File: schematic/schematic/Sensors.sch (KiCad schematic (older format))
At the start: 18 parts, among them J11 Conn_01x07, J12 Conn_01x07, J13 Conn_01x04, J14 Conn_01x04, U10 MPU-9250, U11 MPU-9250, U9 INA219AIDCNR

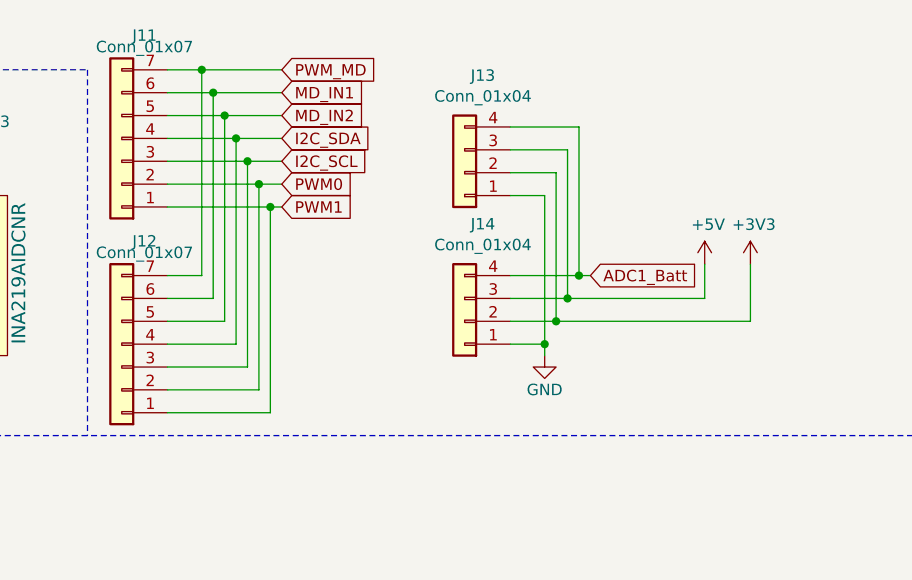
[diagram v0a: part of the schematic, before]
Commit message: 地獄の配線
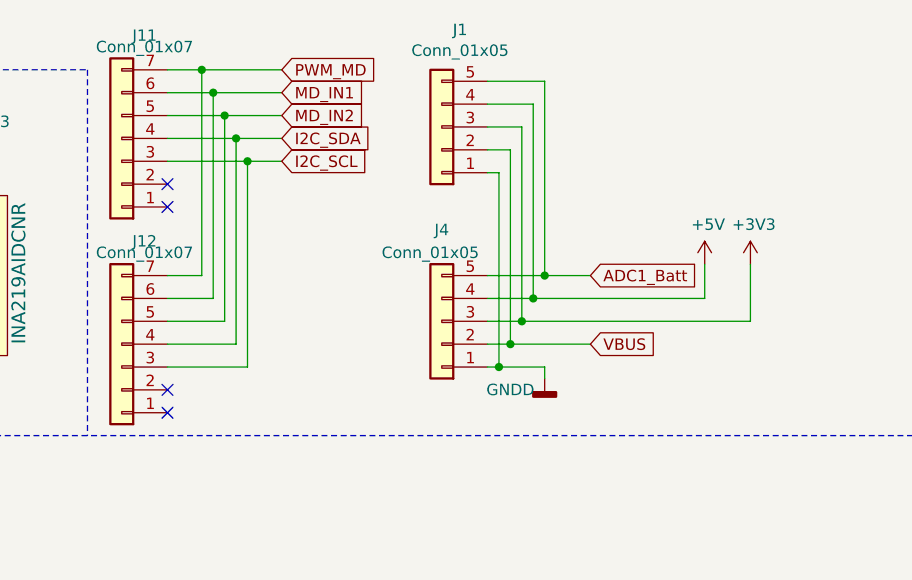
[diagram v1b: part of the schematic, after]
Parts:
- removed J13, J14: Conn_01x04, Connector_PinSocket_2.54mm:PinSocket_1x04_P2.54mm_Vertical, symbol Connector_Generic:Conn_01x04
- added J1, J4: Conn_01x05, Connector_PinHeader_1.00mm:PinHeader_2x03_P1.00mm_Vertical_SMD, symbol Connector_Generic:Conn_01x05
- J11, J12: footprint Connector_PinSocket_2.54mm:PinSocket_1x07_P2.54mm_Vertical -> Connector_PinHeader_1.00mm:PinHeader_2x04_P1.00mm_Vertical_SMD
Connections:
- net +3V3: now also J1.3 (Pin_3), J4.3 (Pin_3)
- net +5V: now also J1.4 (Pin_4), J4.4 (Pin_4)
- net ADC1_Batt: now also J1.5 (Pin_5), J4.5 (Pin_5)
- net GNDD: now also J1.1 (Pin_1), J4.1 (Pin_1)
- net PWM0: no longer names the net of J11.2 (Pin_2)
- net PWM0: no longer J12.2 (Pin_2)
- net PWM1: no longer names the net of J11.1 (Pin_1)
- net PWM1: no longer J12.1 (Pin_1)
- new net VBUS: J1.2 (Pin_2), J4.2 (Pin_2)
- no-connect marks 10 -> 14
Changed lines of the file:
@@
 Text GLabel 3500 1100 2    50   Input ~ 0
 I2C_SCL
-$Comp
-L power:GND #PWR?
-U 1 1 5EC61195
-P 4650 1950
-AR Path="/5EC61195" Ref="#PWR?"  Part="1"
-AR Path="/5E247314/5EC61195" Ref="#PWR075"  Part="1"
-F 0 "#PWR075" H 4650 1700 50  0001 C CNN
-F 1 "GND" H 4650 1800 50  0000 C CNN
-F 2 "" H 4650 1950 50  0001 C CNN
-F 3 "" H 4650 1950 50  0001 C CNN
-	1    4650 1950
-	1    0    0    -1
-$EndComp
 Text GLabel 4850 1600 2    50   Input ~ 0
 ADC1_Batt
 Wire Wire Line
-	4650 1950 4650 1900
-$Comp
-L Connector_Generic:Conn_01x04 J14
-U 1 1 5ECB2FF3
-P 4300 1800
-F 0 "J14" H 4220 1375 50  0000 C CNN
-F 1 "Conn_01x04" H 4220 1466 50  0000 C CNN
-F 2 "Connector_PinSocket_2.54mm:PinSocket_1x04_P2.54mm_Vertical" H 4300 1800 50  0001 C CNN
-F 3 "~" H 4300 1800 50  0001 C CNN
-	1    4300 1800
-	-1   0    0    1
-$EndComp
-$Comp
-L Connector_Generic:Conn_01x04 J13
-U 1 1 5ECB3055
-P 4300 1150
-F 0 "J13" H 4220 725 50  0000 C CNN
-F 1 "Conn_01x04" H 4220 816 50  0000 C CNN
-F 2 "Connector_PinSocket_2.54mm:PinSocket_1x04_P2.54mm_Vertical" H 4300 1150 50  0001 C CNN
-F 3 "~" H 4300 1150 50  0001 C CNN
-	1    4300 1150
-	-1   0    0    1
-$EndComp
-Wire Wire Line
-	4500 1900 4650 1900
+	4650 2050 4650 2000
 $Comp
 L power:+3V3 #PWR077
@@
 	5350 1550 5350 1700
 Wire Wire Line
-	4650 1900 4650 1250
-Wire Wire Line
-	4650 1250 4500 1250
-Connection ~ 4650 1900
-Wire Wire Line
-	4500 1700 4750 1700
-Wire Wire Line
-	4500 1800 4700 1800
-Wire Wire Line
-	4500 1150 4700 1150
-Wire Wire Line
-	4700 1150 4700 1800
-Connection ~ 4700 1800
-Wire Wire Line
-	4500 1050 4750 1050
-Wire Wire Line
-	4750 1050 4750 1700
-Connection ~ 4750 1700
-Wire Wire Line
 	5550 1550 5550 1800
-Wire Wire Line
-	4750 1700 5350 1700
-Wire Wire Line
-	4700 1800 5550 1800
-Wire Wire Line
-	4500 950  4800 950
-Wire Wire Line
-	4800 950  4800 1600
-Wire Wire Line
-	4800 1600 4500 1600
-Wire Wire Line
-	4850 1600 4800 1600
-Connection ~ 4800 1600
-Text GLabel 3500 1200 2    50   Input ~ 0
-PWM0
-Text GLabel 3500 1300 2    50   Input ~ 0
-PWM1
 $Comp
 L Connector_Generic:Conn_01x07 J11
@@
 F 0 "J11" H 2700 550 50  0000 C CNN
 F 1 "Conn_01x07" H 2700 600 50  0000 C CNN
-F 2 "Connector_PinSocket_2.54mm:PinSocket_1x07_P2.54mm_Vertical" H 2800 1000 50  0001 C CNN
+F 2 "Connector_PinHeader_1.00mm:PinHeader_2x04_P1.00mm_Vertical_SMD" H 2800 1000 50  0001 C CNN
 F 3 "~" H 2800 1000 50  0001 C CNN
 	1    2800 1000
@@
 F 0 "J12" H 2700 1450 50  0000 C CNN
 F 1 "Conn_01x07" H 2700 1500 50  0000 C CNN
-F 2 "Connector_PinSocket_2.54mm:PinSocket_1x07_P2.54mm_Vertical" H 2800 1900 50  0001 C CNN
+F 2 "Connector_PinHeader_1.00mm:PinHeader_2x04_P1.00mm_Vertical_SMD" H 2800 1900 50  0001 C CNN
 F 3 "~" H 2800 1900 50  0001 C CNN
 	1    2800 1900
@@
 	3000 1100 3350 1100
 Wire Wire Line
-	3000 1200 3400 1200
-Wire Wire Line
 	3000 1600 3150 1600
 Wire Wire Line
@@
 Connection ~ 3350 1100
 Wire Wire Line
-	3400 1200 3400 2100
-Wire Wire Line
-	3400 2100 3000 2100
-Connection ~ 3400 1200
-Wire Wire Line
-	3000 1300 3450 1300
-Wire Wire Line
-	3400 1200 3500 1200
-Wire Wire Line
 	3350 1100 3500 1100
 Wire Wire Line
@@
 Wire Wire Line
 	3150 700  3500 700
-Wire Wire Line
-	3450 1300 3450 2200
-Wire Wire Line
-	3450 2200 3000 2200
-Connection ~ 3450 1300
-Wire Wire Line
-	3450 1300 3500 1300
 $Comp
 L Device:R_Small R29
@@
 	1    0    0    -1
 $EndComp
+$Comp
+L Connector_Generic:Conn_01x05 J4
+U 1 1 5EF1C02F
+P 4200 1800
+F 0 "J4" H 4200 1400 50  0000 C CNN
+F 1 "Conn_01x05" H 4250 1500 50  0000 C CNN
+F 2 "Connector_PinHeader_1.00mm:PinHeader_2x03_P1.00mm_Vertical_SMD" H 4200 1800 50  0001 C CNN
+F 3 "~" H 4200 1800 50  0001 C CNN
+	1    4200 1800
+	-1   0    0    1
+$EndComp
+Wire Wire Line
+	4400 1600 4650 1600
+Wire Wire Line
+	4400 1700 4600 1700
+Wire Wire Line
+	4400 1800 4550 1800
+Wire Wire Line
+	4400 1900 4500 1900
+Wire Wire Line
+	4400 2000 4450 2000
+$Comp
+L Connector_Generic:Conn_01x05 J1
+U 1 1 5EF40D9B
+P 4200 950
+F 0 "J1" H 4120 525 50  0000 C CNN
+F 1 "Conn_01x05" H 4120 616 50  0000 C CNN
+F 2 "Connector_PinHeader_1.00mm:PinHeader_2x03_P1.00mm_Vertical_SMD" H 4200 950 50  0001 C CNN
+F 3 "~" H 4200 950 50  0001 C CNN
+	1    4200 950
+	-1   0    0    1
+$EndComp
+Wire Wire Line
+	4400 1150 4450 1150
+Wire Wire Line
+	4450 1150 4450 2000
+Connection ~ 4450 2000
+Wire Wire Line
+	4450 2000 4650 2000
+Wire Wire Line
+	4500 1900 4500 1050
+Wire Wire Line
+	4500 1050 4400 1050
+Connection ~ 4500 1900
+Wire Wire Line
+	4500 1900 4850 1900
+Wire Wire Line
+	4400 950  4550 950
+Wire Wire Line
+	4550 950  4550 1800
+Connection ~ 4550 1800
+Wire Wire Line
+	4550 1800 5550 1800
+Wire Wire Line
+	4600 1700 4600 850
+Wire Wire Line
+	4600 850  4400 850
+Connection ~ 4600 1700
+Wire Wire Line
+	4600 1700 5350 1700
+Wire Wire Line
+	4400 750  4650 750
+Wire Wire Line
+	4650 750  4650 1600
+Connection ~ 4650 1600
+Wire Wire Line
+	4650 1600 4850 1600
+Text GLabel 4850 1900 2    50   Input ~ 0
+VBUS
+$Comp
+L power:GNDD #PWR?
+U 1 1 5EF5FD4C
+P 4650 2050
+AR Path="/5EF5FD4C" Ref="#PWR?"  Part="1"
+AR Path="/5E247314/5EF5FD4C" Ref="#PWR0101"  Part="1"
+F 0 "#PWR0101" H 4650 1800 50  0001 C CNN
+F 1 "GNDD" H 4500 2000 50  0000 C CNN
+F 2 "" H 4650 2050 50  0001 C CNN
+F 3 "" H 4650 2050 50  0001 C CNN
+	1    4650 2050
+	1    0    0    -1
+$EndComp
+NoConn ~ 3000 2100
+NoConn ~ 3000 2200
+NoConn ~ 3000 1300
+NoConn ~ 3000 1200
 Wire Bus Line
 	1550 5550 1550 5950

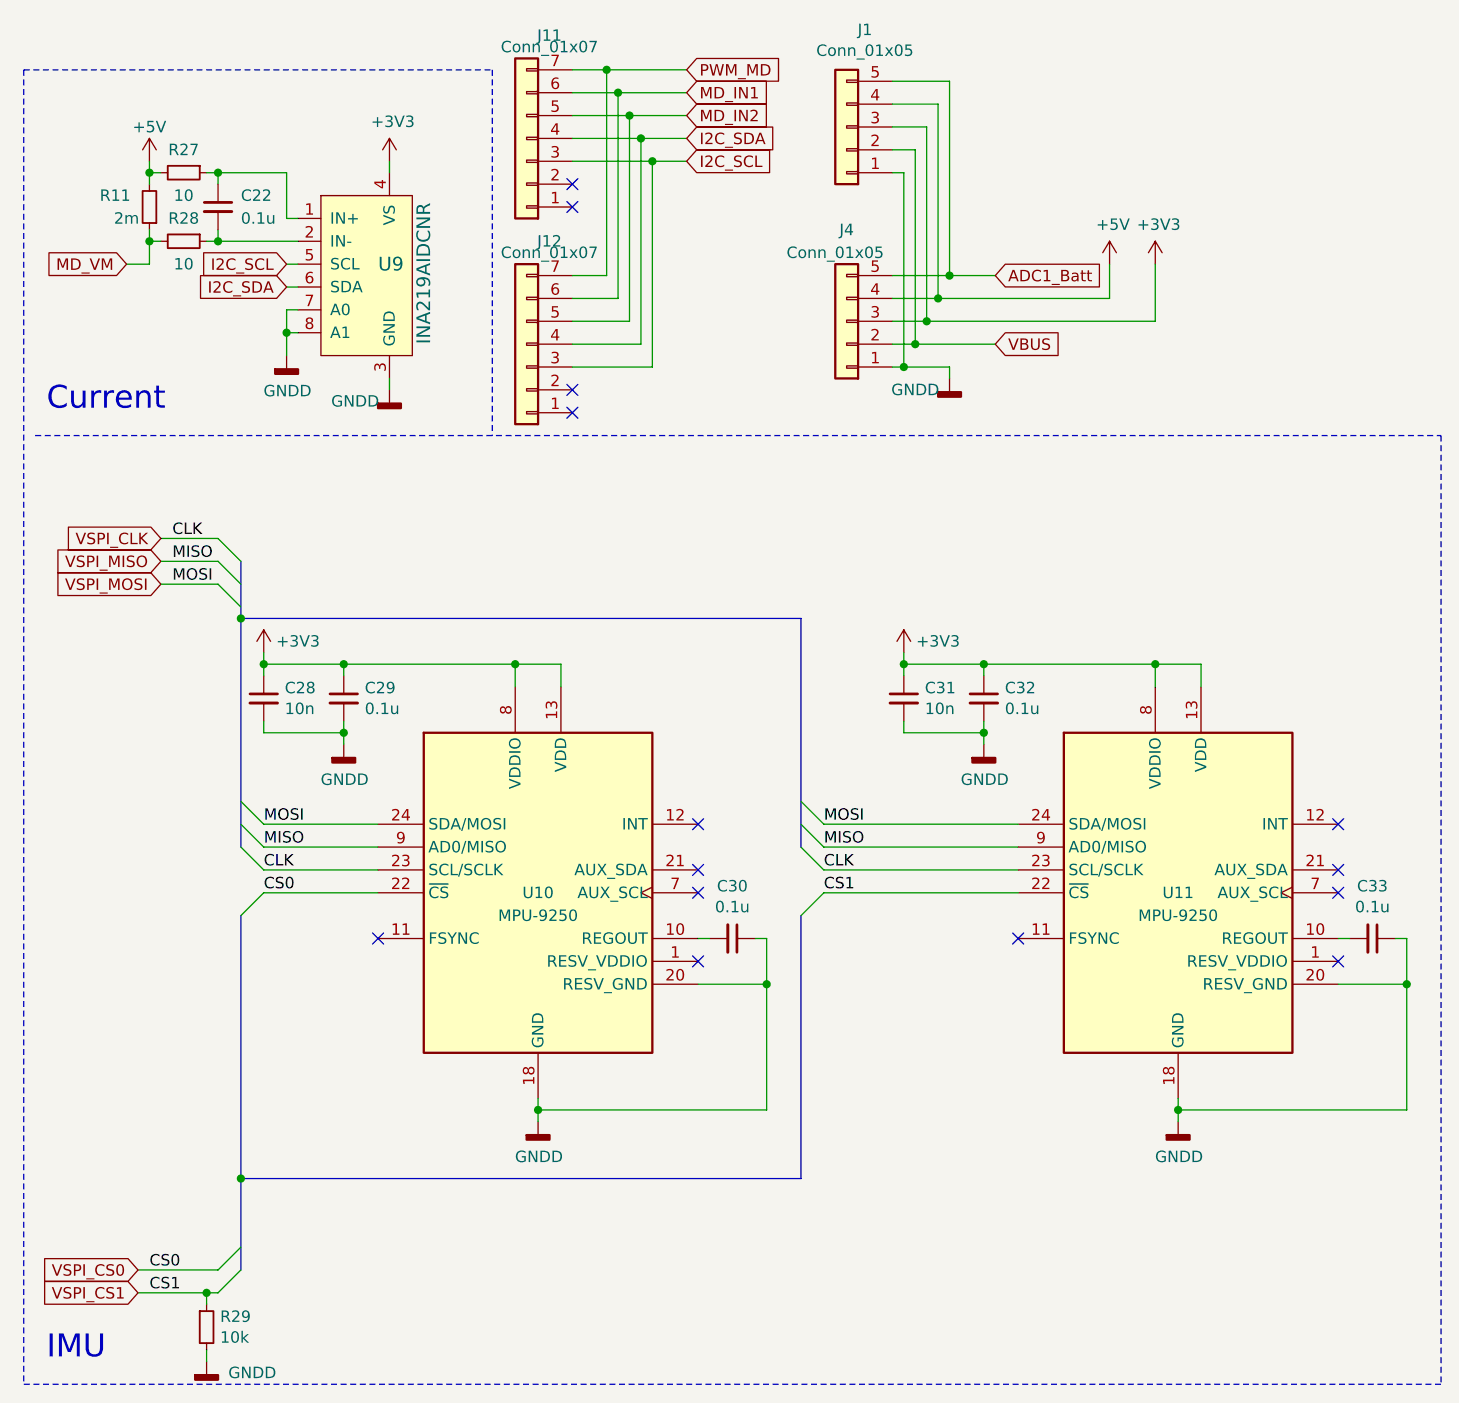
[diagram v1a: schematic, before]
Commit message: 一歩進んで仕様決めなおし
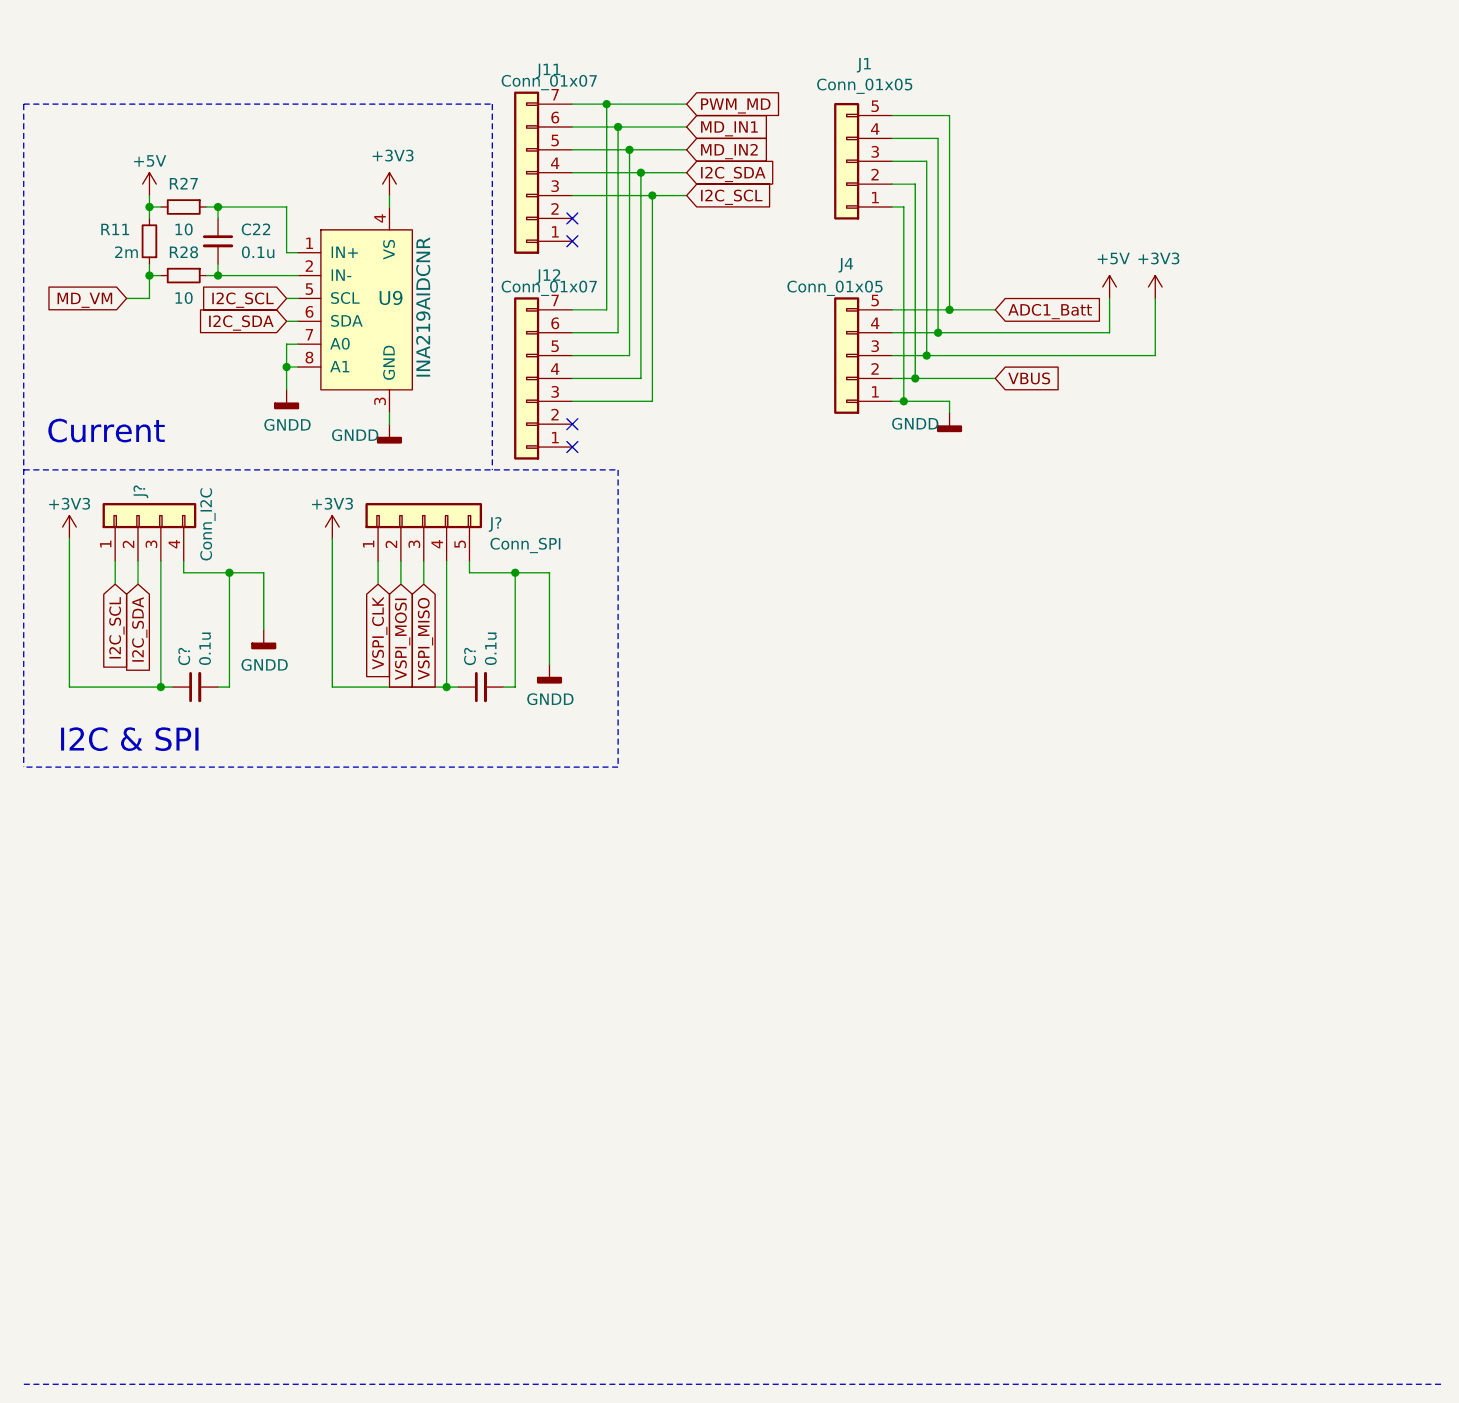
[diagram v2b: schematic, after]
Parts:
- removed C28, C31: 10n, micelib:C_0201_0603Metric_HandSoldering, symbol Device:C_Small
- removed C29, C30, C32, C33: 0.1u, micelib:C_0402_1005Metric_HandSoldering, symbol Device:C_Small
- removed R29: 10k, micelib:C_0402_1005Metric_HandSoldering, symbol Device:R_Small
- removed U10, U11: MPU-9250, micelib:InvenSense_QFN-24_3x3mm_P0.4mm_HandSoldering, symbol Sensor_Motion:MPU-9250
- added C? (x2): 0.1u, micelib:C_0402_1005Metric_HandSoldering, symbol Device:C_Small
- added J?: Conn_I2C, Connector_PinHeader_2.54mm:PinHeader_1x04_P2.54mm_Vertical, symbol Connector_Generic:Conn_01x04
- added J?: Conn_SPI, symbol Connector_Generic:Conn_01x05
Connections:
- net +3V3: now also C?.1, C?.1, J?.3 (Pin_3), J?.4 (Pin_4)
- net GNDD: now also C?.2, C?.2, J?.4 (Pin_4), J?.5 (Pin_5)
- net I2C_SCL: now also J?.1 (Pin_1)
- net I2C_SDA: now also J?.2 (Pin_2)
- net VSPI_CLK: now also J?.1 (Pin_1)
- net VSPI_MISO: now also J?.3 (Pin_3)
- net VSPI_MOSI: now also J?.2 (Pin_2)
- no-connect marks 14 -> 4
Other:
- note added: "I2C & SPI"
- note removed: "IMU"
- moved on the sheet: C22, J1, J11, J12, J4, R11, R27, R28, U9
